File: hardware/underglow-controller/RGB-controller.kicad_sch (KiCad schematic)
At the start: 0 parts

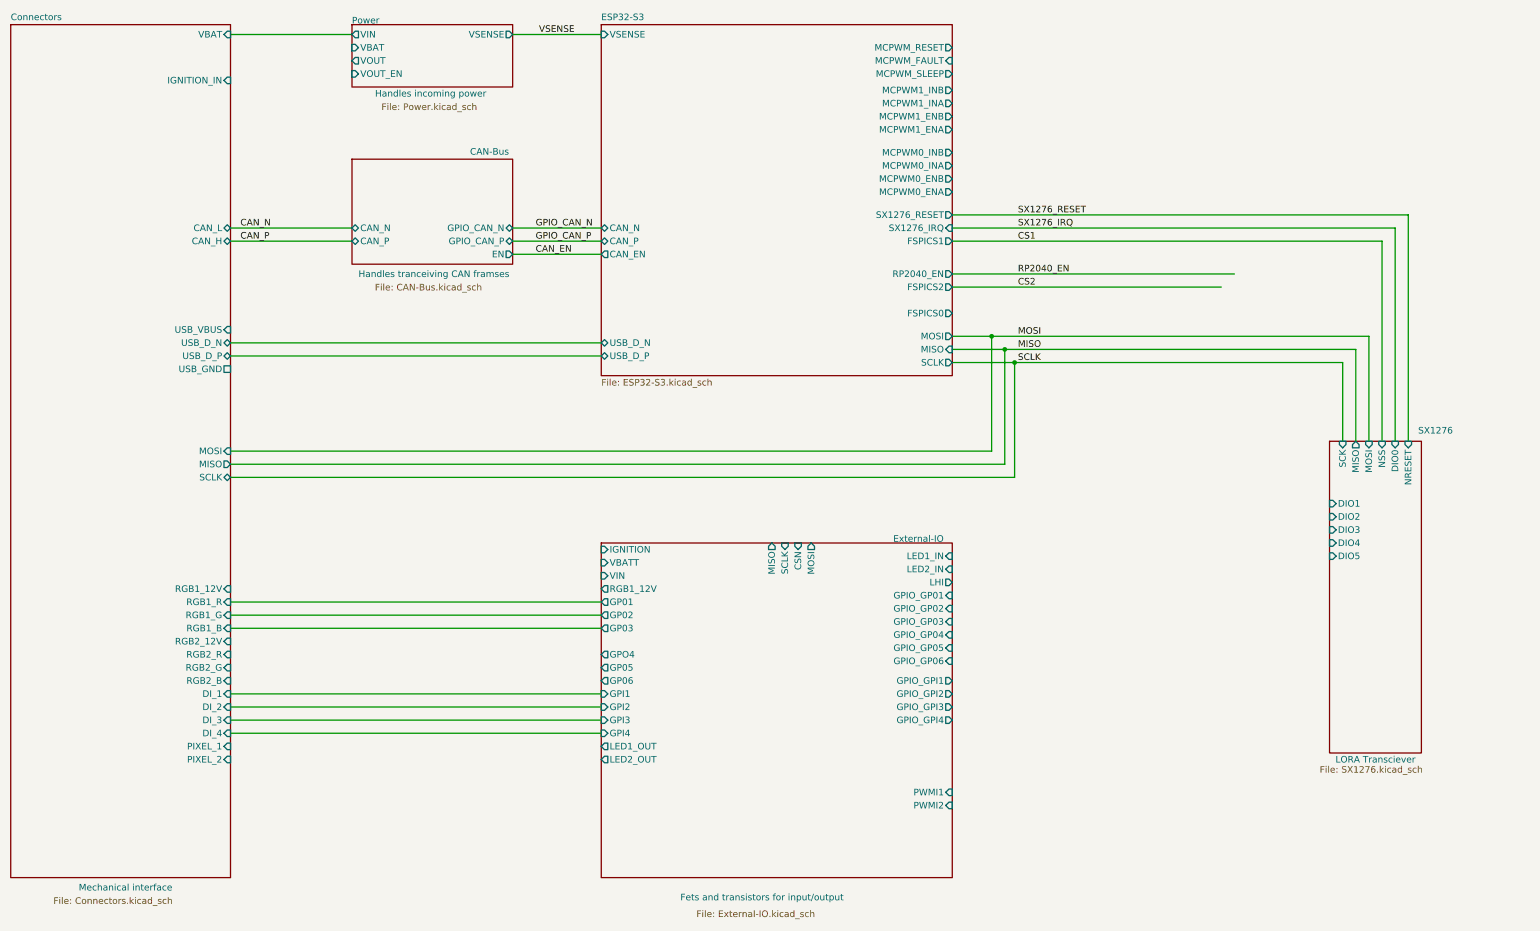
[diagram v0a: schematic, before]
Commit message: schematic almost done
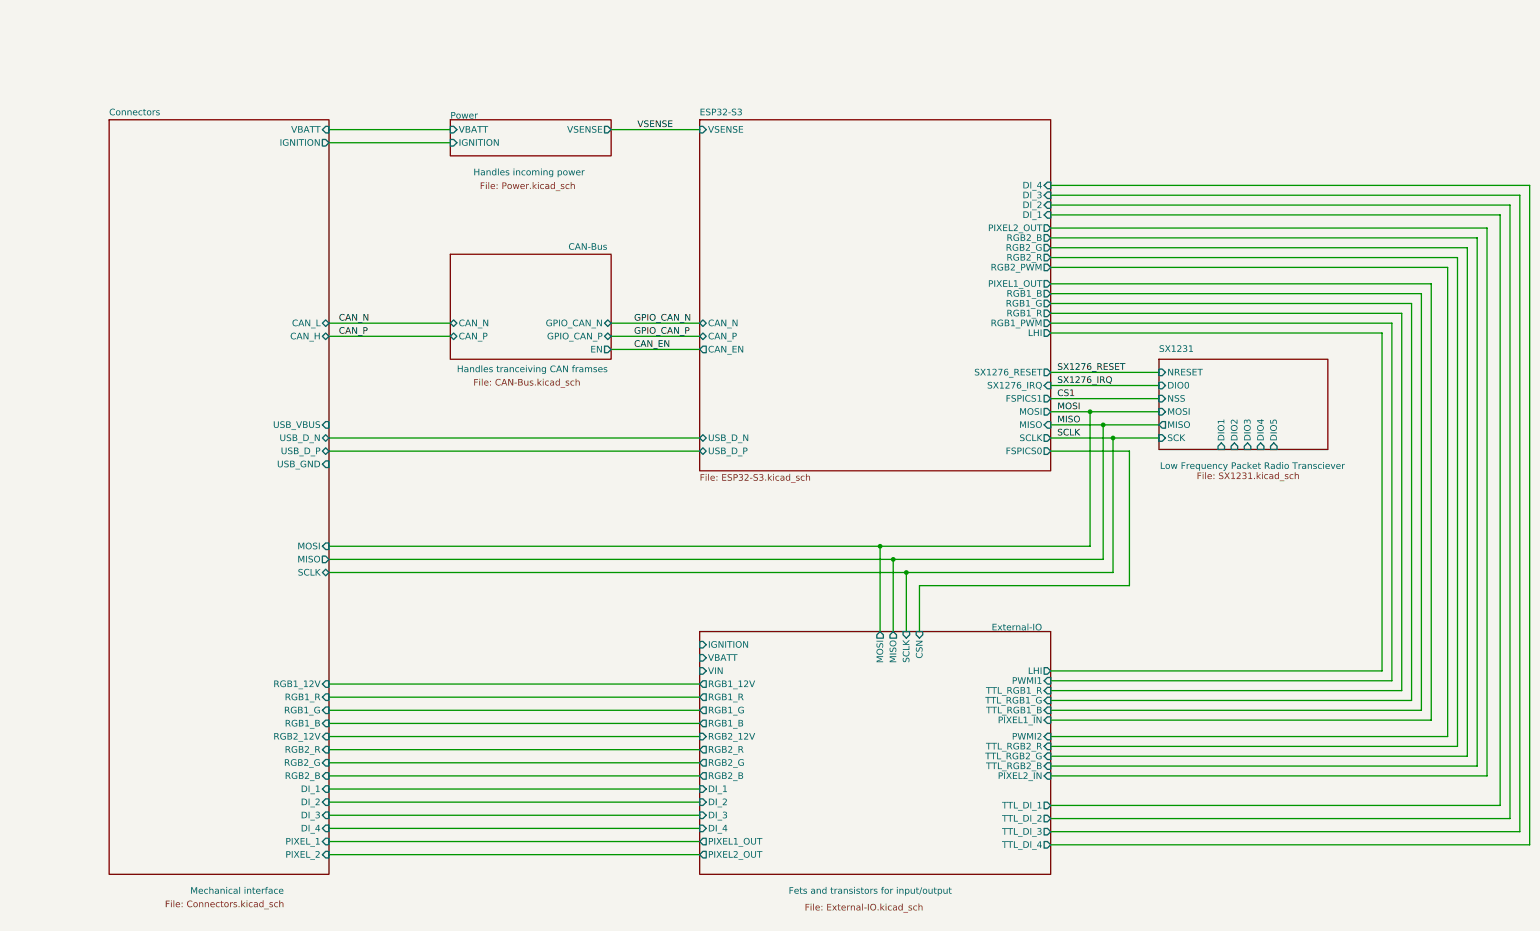
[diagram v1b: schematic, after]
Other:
- sheet SX1276 renamed SX1231
- sheet Connectors ports: added IGNITION, VBATT; removed IGNITION_IN, VBAT
- sheet ESP32-S3 ports: added DI_1, DI_2, DI_3, DI_4, LHI, PIXEL1_OUT, PIXEL2_OUT, RGB1_B, RGB1_G, RGB1_PWM, RGB1_R, RGB2_B, RGB2_G, RGB2_PWM, RGB2_R; removed FSPICS2, MCPWM0_ENA, MCPWM0_ENB, MCPWM0_INA, MCPWM0_INB, MCPWM1_ENA, MCPWM1_ENB, MCPWM1_INA, MCPWM1_INB, MCPWM_FAULT, MCPWM_RESET, MCPWM_SLEEP, RP2040_EN
- sheet External-IO ports: added DI_1, DI_2, DI_3, DI_4, PIXEL1_IN, PIXEL1_OUT, PIXEL2_IN, PIXEL2_OUT, RGB1_B, RGB1_G, RGB1_R, RGB2_12V, RGB2_B, RGB2_G, RGB2_R, TTL_DI_1, TTL_DI_2, TTL_DI_3, TTL_DI_4, TTL_RGB1_B, TTL_RGB1_G, TTL_RGB1_R, TTL_RGB2_B, TTL_RGB2_G, TTL_RGB2_R; removed GP01, GP02, GP03, GP05, GP06, GPI1, GPI2, GPI3, GPI4, GPIO_GP01, GPIO_GP02, GPIO_GP03, GPIO_GP04, GPIO_GP05, GPIO_GP06, GPIO_GPI1, GPIO_GPI2, GPIO_GPI3, GPIO_GPI4, GPO4, LED1_IN, LED1_OUT, LED2_IN, LED2_OUT
- sheet Power ports: added IGNITION, VBATT; removed VBAT, VIN, VOUT, VOUT_EN
- sheet SX1231: file SX1276.kicad_sch -> SX1231.kicad_sch
